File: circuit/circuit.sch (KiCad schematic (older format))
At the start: 25 parts, among them J1 USB, J2 Conn_01x05_Male, J3 STEPPER, J5 LEDS, SW1 S_MODE, U1 TSR12450, U2 Feather, U3 4N35, U4 L293D

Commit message: Stuff
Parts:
- removed U1: TSR12450, Footprints:TSR1, symbol Gauge-rescue:TSR12450-New_Library
- removed U2: Feather, Footprints:Feather, symbol Gauge-rescue:Feather-New_Library
- removed U4: L293D, Footprints:L293D, symbol Gauge-rescue:L293D-New_Library
- added U?: TSR12450, symbol library:TSR12450
- added U?: L293D, symbol library:L293D
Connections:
- wire segments 96 -> 95
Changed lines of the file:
@@
 EESchema Schematic File Version 4
-LIBS:Gauge-cache
 EELAYER 26 0
 EELAYER END
@@
 $EndDescr
 $Comp
-L Gauge-rescue:L293D-New_Library U4
-U 1 1 5CB8E603
-P 8450 5050
-F 0 "U4" H 9028 5096 50  0000 L CNN
-F 1 "L293D" H 9028 5005 50  0000 L CNN
-F 2 "Footprints:L293D" H 8350 5050 50  0001 C CNN
-F 3 "" H 8350 5050 50  0001 C CNN
-	1    8450 5050
-	1    0    0    -1
-$EndComp
-$Comp
 L LED:CQY99 D4
 U 1 1 5CB8F18D
@@
 	1    0    0    -1
 $EndComp
-Wire Wire Line
-	8500 5650 8350 5650
-Connection ~ 8350 5650
 $Comp
 L power:GND #PWR0124
@@
 	8350 4350 7500 4350
 Connection ~ 8350 4350
-$Comp
-L Gauge-rescue:Feather-New_Library U2
-U 1 1 5CBFD77E
-P 3450 5850
-F 0 "U2" H 3450 6865 50  0000 C CNN
-F 1 "Feather" H 3450 6774 50  0000 C CNN
-F 2 "Footprints:Feather" H 3450 5850 50  0001 C CNN
-F 3 "" H 3450 5850 50  0001 C CNN
-	1    3450 5850
-	1    0    0    -1
-$EndComp
 Wire Wire Line
 	3900 5700 4100 5700
-$Comp
-L Gauge-rescue:TSR12450-New_Library U1
-U 1 1 5CC457F0
-P 2100 3450
-F 0 "U1" H 2100 3775 50  0000 C CNN
-F 1 "TSR12450" H 2100 3684 50  0000 C CNN
-F 2 "Footprints:TSR1" H 2100 3450 50  0001 C CNN
-F 3 "" H 2100 3450 50  0001 C CNN
-	1    2100 3450
-	1    0    0    -1
-$EndComp
 $Comp
 L Connector:Conn_01x04_Male J5
@@
 $EndComp
 Connection ~ 6350 1300
+$Comp
+L library:TSR12450 U?
+U 1 1 5CC85FA4
+P 2100 3450
+F 0 "U?" H 2100 3775 50  0000 C CNN
+F 1 "TSR12450" H 2100 3684 50  0000 C CNN
+F 2 "" H 2100 3450 50  0001 C CNN
+F 3 "" H 2100 3450 50  0001 C CNN
+	1    2100 3450
+	1    0    0    -1
+$EndComp
+$Comp
+L library:L293D U?
+U 1 1 5CC8619E
+P 8450 5050
+F 0 "U?" H 9028 5096 50  0000 L CNN
+F 1 "L293D" H 9028 5005 50  0000 L CNN
+F 2 "" H 8350 5050 50  0001 C CNN
+F 3 "" H 8350 5050 50  0001 C CNN
+	1    8450 5050
+	1    0    0    -1
+$EndComp
 $EndSCHEMATC

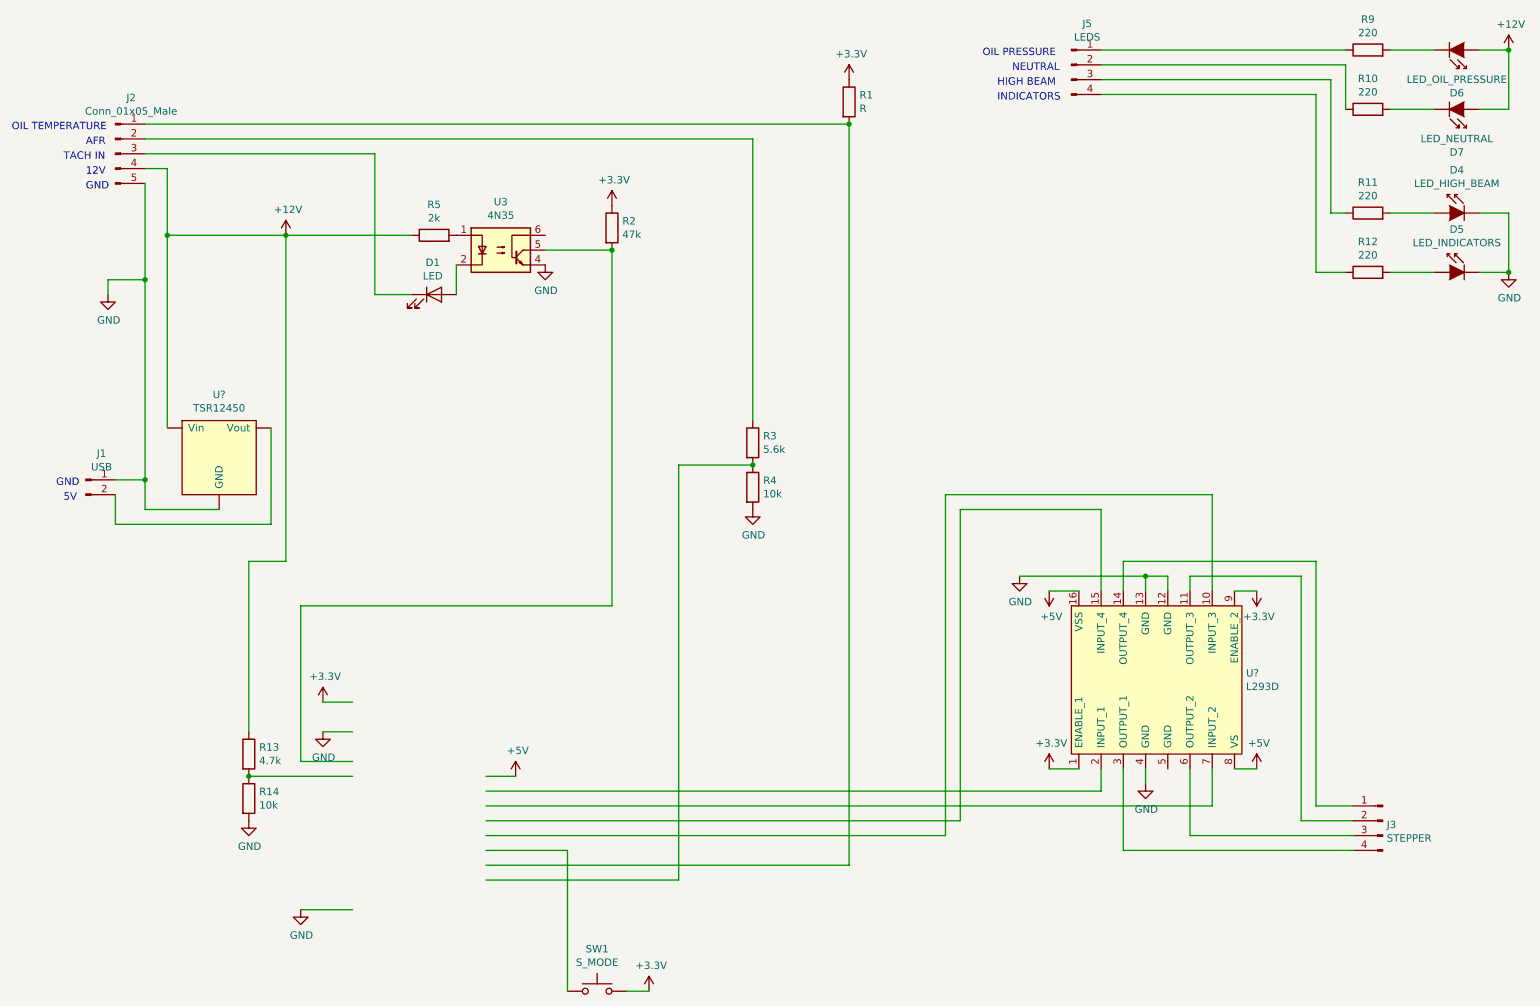
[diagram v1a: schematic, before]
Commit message: Stuff
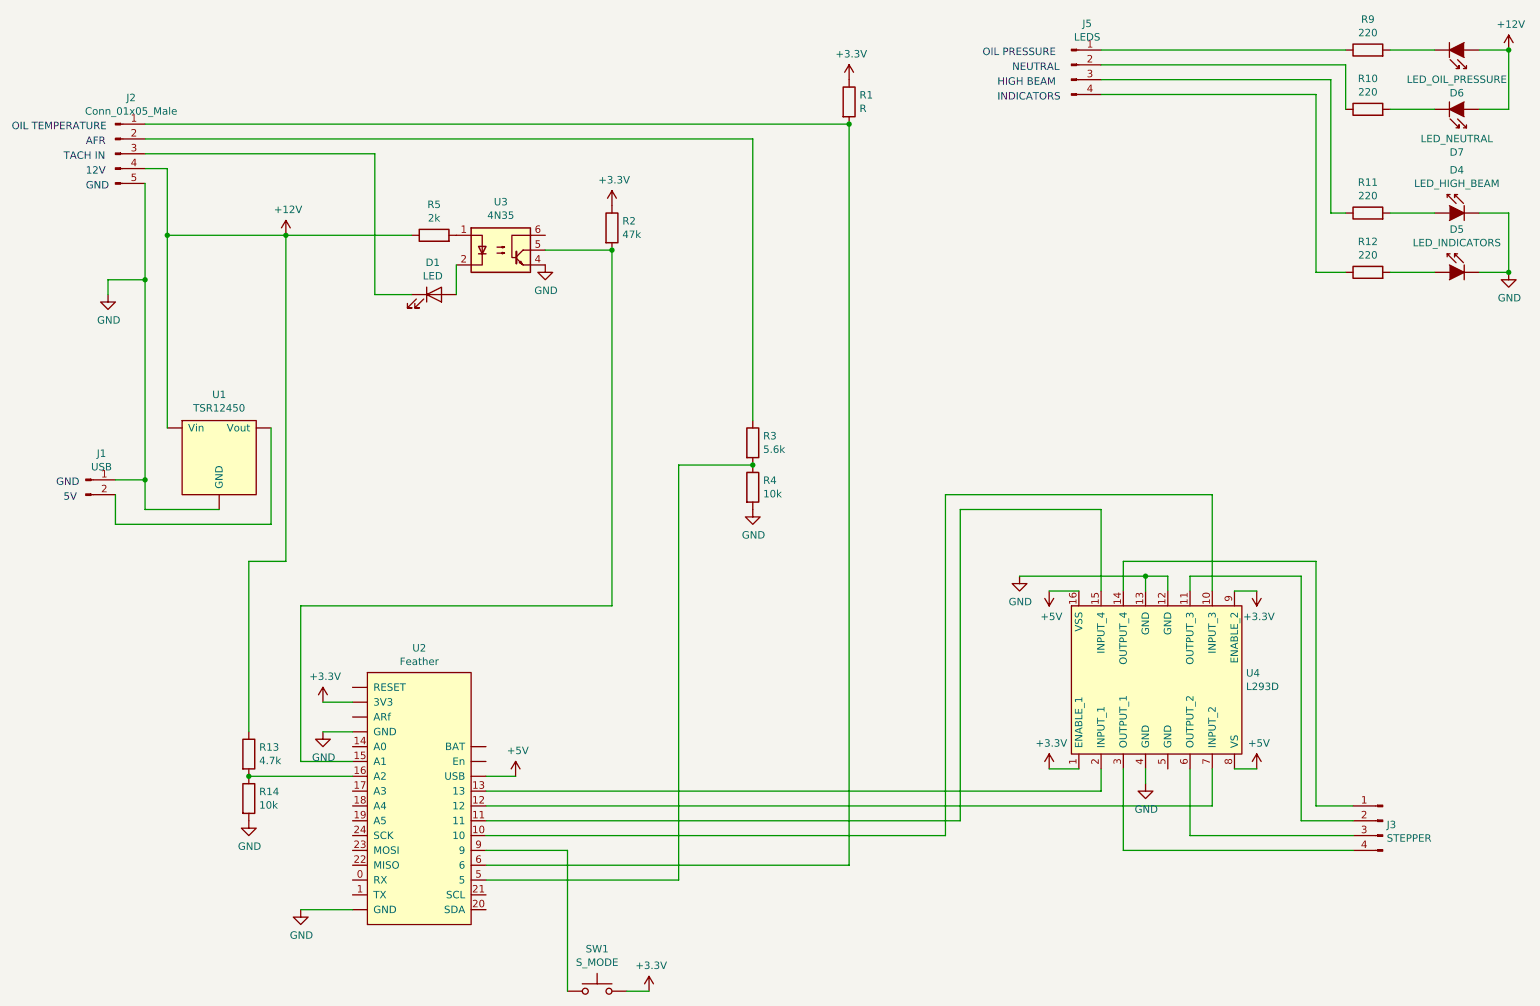
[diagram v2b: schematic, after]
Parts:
- added U2: Feather, Footprints:Feather, symbol library:Feather
- U1: renamed from U?; footprint (none) -> Footprints:TSR1
- U4: renamed from U?; footprint (none) -> Footprints:L293D
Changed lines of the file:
@@
 EESchema Schematic File Version 4
+LIBS:circuit-cache
 EELAYER 26 0
 EELAYER END
@@
 Connection ~ 6350 1300
 $Comp
-L library:TSR12450 U?
+L library:TSR12450 U1
 U 1 1 5CC85FA4
 P 2100 3450
-F 0 "U?" H 2100 3775 50  0000 C CNN
+F 0 "U1" H 2100 3775 50  0000 C CNN
 F 1 "TSR12450" H 2100 3684 50  0000 C CNN
-F 2 "" H 2100 3450 50  0001 C CNN
+F 2 "Footprints:TSR1" H 2100 3450 50  0001 C CNN
 F 3 "" H 2100 3450 50  0001 C CNN
 	1    2100 3450
@@
 $EndComp
 $Comp
-L library:L293D U?
+L library:L293D U4
 U 1 1 5CC8619E
 P 8450 5050
-F 0 "U?" H 9028 5096 50  0000 L CNN
+F 0 "U4" H 9028 5096 50  0000 L CNN
 F 1 "L293D" H 9028 5005 50  0000 L CNN
-F 2 "" H 8350 5050 50  0001 C CNN
+F 2 "Footprints:L293D" H 8350 5050 50  0001 C CNN
 F 3 "" H 8350 5050 50  0001 C CNN
 	1    8450 5050
 	1    0    0    -1
 $EndComp
+$Comp
+L library:Feather U2
+U 1 1 5CCEA291
+P 3450 5850
+F 0 "U2" H 3450 6865 50  0000 C CNN
+F 1 "Feather" H 3450 6774 50  0000 C CNN
+F 2 "Footprints:Feather" H 3450 5850 50  0001 C CNN
+F 3 "" H 3450 5850 50  0001 C CNN
+	1    3450 5850
+	1    0    0    -1
+$EndComp

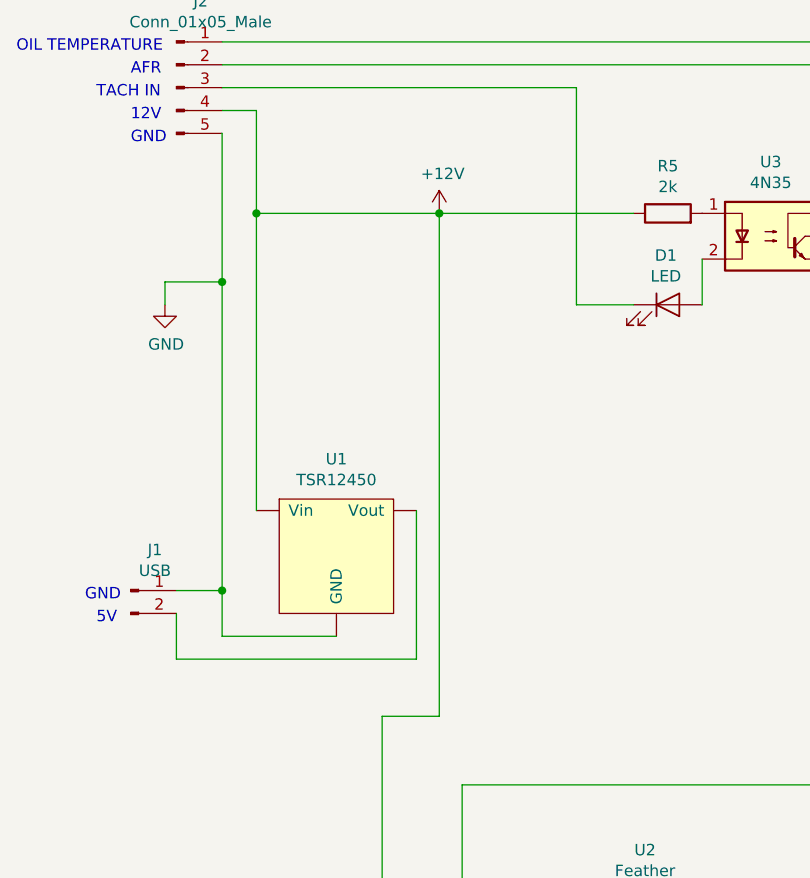
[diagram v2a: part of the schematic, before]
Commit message: Stuff
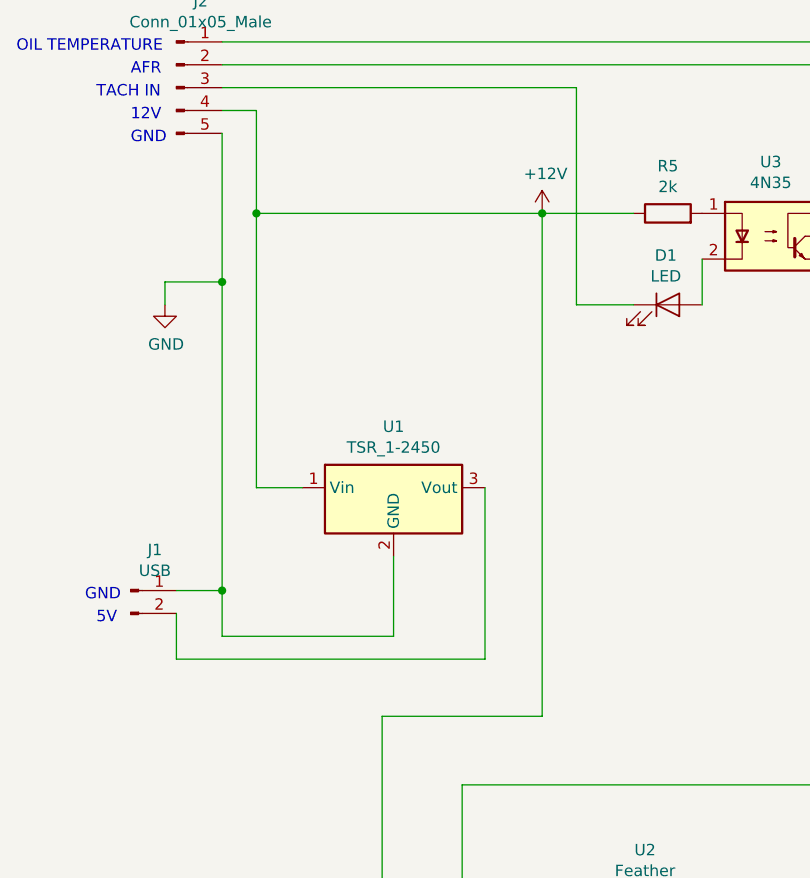
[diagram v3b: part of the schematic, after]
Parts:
- removed U1: TSR12450, Footprints:TSR1, symbol library:TSR12450
- added U1: TSR_1-2450, Converter_DCDC:Converter_DCDC_TRACO_TSR-1_THT, symbol Regulator_Switching:TSR_1-2450
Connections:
- net +12V: now also U1.1 (Vin)
- net GND: now also U1.2 (GND)
- net at J1.2 (Pin_2): now also U1.3 (Vout)
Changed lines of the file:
@@
 $EndComp
-Wire Wire Line
-	2100 3900 1600 3900
 Wire Wire Line
 	1600 3900 1600 3700
-Wire Wire Line
-	2450 3350 2450 4000
-Wire Wire Line
-	2450 4000 1400 4000
 Wire Wire Line
 	1400 4000 1400 3800
@@
 Connection ~ 1750 2050
 Wire Wire Line
-	1750 2050 1750 3350
+	1750 2050 1750 3250
 $Comp
 L Switch:SW_Push SW1
@@
 L power:+12V #PWR0114
 U 1 1 5CBD1F19
-P 2550 2050
-F 0 "#PWR0114" H 2550 1900 50  0001 C CNN
-F 1 "+12V" H 2565 2223 50  0000 C CNN
-F 2 "" H 2550 2050 50  0001 C CNN
-F 3 "" H 2550 2050 50  0001 C CNN
-	1    2550 2050
+P 3000 2050
+F 0 "#PWR0114" H 3000 1900 50  0001 C CNN
+F 1 "+12V" H 3015 2223 50  0000 C CNN
+F 2 "" H 3000 2050 50  0001 C CNN
+F 3 "" H 3000 2050 50  0001 C CNN
+	1    3000 2050
 	1    0    0    -1
 $EndComp
@@
 Wire Wire Line
 	2300 5400 2300 4250
-Wire Wire Line
-	2300 4250 2550 4250
-Wire Wire Line
-	2550 4250 2550 2050
-Connection ~ 2550 2050
-Wire Wire Line
-	1750 2050 2550 2050
 $Comp
 L Connector:Conn_01x05_Male J2
@@
 $EndComp
 Wire Wire Line
-	3400 2050 2550 2050
+	3400 2050 3000 2050
 $Comp
 L Device:LED D1
@@
 Connection ~ 6350 1300
 $Comp
-L library:TSR12450 U1
-U 1 1 5CC85FA4
-P 2100 3450
-F 0 "U1" H 2100 3775 50  0000 C CNN
-F 1 "TSR12450" H 2100 3684 50  0000 C CNN
-F 2 "Footprints:TSR1" H 2100 3450 50  0001 C CNN
-F 3 "" H 2100 3450 50  0001 C CNN
-	1    2100 3450
-	1    0    0    -1
-$EndComp
-$Comp
 L library:L293D U4
 U 1 1 5CC8619E
@@
 	1    0    0    -1
 $EndComp
+Wire Wire Line
+	3000 4250 3000 2050
+Wire Wire Line
+	2300 4250 3000 4250
+Connection ~ 3000 2050
+Wire Wire Line
+	1750 2050 3000 2050
+$Comp
+L Regulator_Switching:TSR_1-2450 U1
+U 1 1 5CD33323
+P 2350 3350
+F 0 "U1" H 2350 3717 50  0000 C CNN
+F 1 "TSR_1-2450" H 2350 3626 50  0000 C CNN
+F 2 "Converter_DCDC:Converter_DCDC_TRACO_TSR-1_THT" H 2350 3200 50  0001 L CIN
+F 3 "http://www.tracopower.com/products/tsr1.pdf" H 2350 3350 50  0001 C CNN
+	1    2350 3350
+	1    0    0    -1
+$EndComp
+Wire Wire Line
+	2750 4000 2750 3250
+Wire Wire Line
+	1400 4000 2750 4000
+Wire Wire Line
+	2350 3900 2350 3550
+Wire Wire Line
+	1600 3900 2350 3900
+Wire Wire Line
+	1950 3250 1750 3250
 $EndSCHEMATC
